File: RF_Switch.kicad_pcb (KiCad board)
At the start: 2 copper layers, 38.1 x 38.1 mm, 5 parts, among them J1 Conn_Coaxial, J2 Conn_01x04, J3 Conn_Coaxial, J4 Conn_Coaxial, U1 HSWA2-30DR+

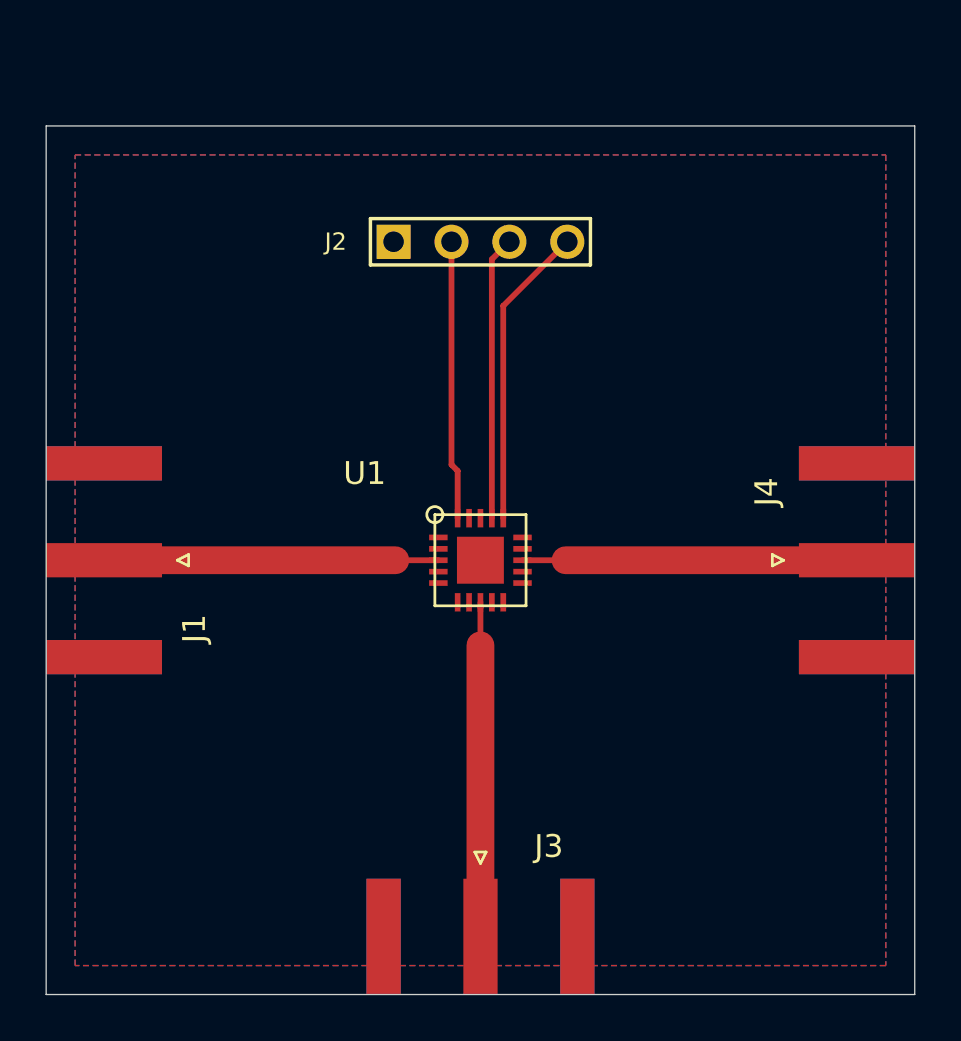
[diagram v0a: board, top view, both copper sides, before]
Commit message: Finished REV A
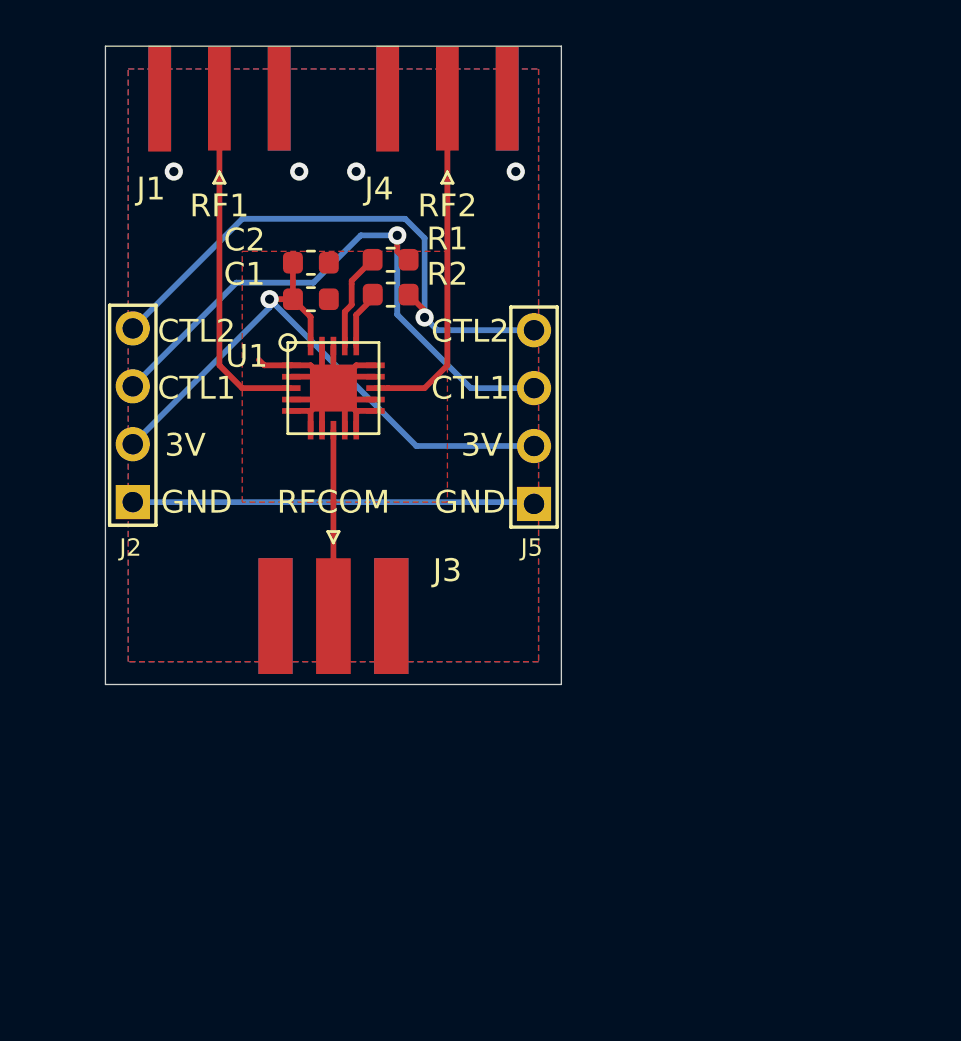
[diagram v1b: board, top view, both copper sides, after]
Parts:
- added C1: 100pF, Capacitor_SMD:C_0603_1608Metric, F.Cu at (164.0, 71.1)
- added C2: 0.1uF, Capacitor_SMD:C_0603_1608Metric, F.Cu at (164.0, 69.5)
- added J5: Conn_01x04, lib_fp:Header 4 Keyed RT Angle, F.Cu at (173.8, 80.1)
- added R1: 4.7k, Resistor_SMD:R_0603_1608Metric, F.Cu at (167.5, 69.4)
- added R2: 4.7k, Resistor_SMD:R_0603_1608Metric, F.Cu at (167.5, 70.9)
- J1, J4: footprint Connector_Coaxial:SMA_Amphenol_132289_EdgeMount -> lib_fp:SMA_Taoglas_Limited_Narrow_EdgeMount
- J3: footprint Connector_Coaxial:SMA_Amphenol_132289_EdgeMount -> lib_fp:SMA_Plug_Linx_Technologies_EdgeMount_CONSMA013.062
- moved J4 27.1 mm to (170.0, 62.3), turned to 90 degrees
- moved J1 20.9 mm to (160.0, 62.3), turned to 90 degrees
- moved J2 16.2 mm to (156.2, 80.0), turned to 0 degrees
- moved J3 15.5 mm to (165.0, 85.0)
- moved U1 9.93 mm to (165.0, 75.0)
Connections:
- U1 pad 15: (no net) -> GND
- U1 pad 16: Net-(J2-Pad4) -> Net-(R2-Pad2)
- U1 pad 17: Net-(J2-Pad3) -> Net-(R1-Pad2)
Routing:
- net GND: track 0.00 -> 44.0 mm, vias 0 -> 4
- net Net-(C1-Pad1): track 12.2 -> 28.1 mm, vias 0 -> 1
- net Net-(J2-Pad3): track 12.4 -> 26.5 mm, vias 0 -> 1
- net Net-(J2-Pad4): track 13.3 -> 24.9 mm, vias 0 -> 1
- net Net-(J3-Pad1): track 14.1 -> 8.16 mm
- net Net-(R1-Pad2): track 0.00 -> 4.29 mm
- net Net-(R2-Pad2): track 0.00 -> 2.56 mm
- net Net-(J1-Pad1): track 14.1 -> 15.3 mm
- net Net-(J4-Pad1): track 14.1 -> 15.3 mm
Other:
- board size 38.1 x 38.1 mm -> 20 x 28 mm
- board text added: "3V"
- board text added: "CTL1"
- board text added: "CTL2"
- board text added: "GND"
- board text added: "RF1"
- board text added: "RF2"
- board text added: "RFCOM"
